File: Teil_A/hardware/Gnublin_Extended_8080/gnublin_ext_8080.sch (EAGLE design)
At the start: 7 parts

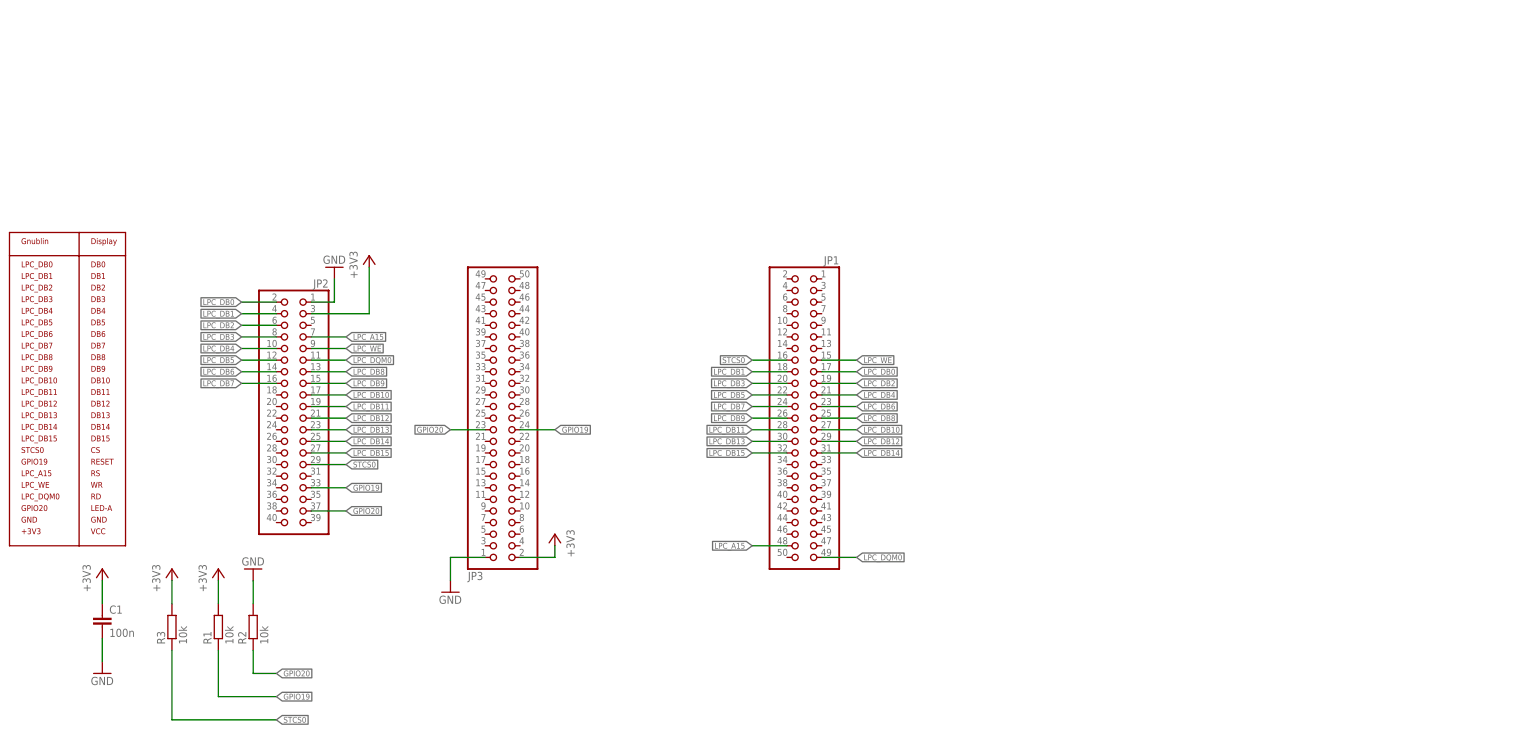
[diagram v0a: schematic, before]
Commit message: end of workday 29.07.2014
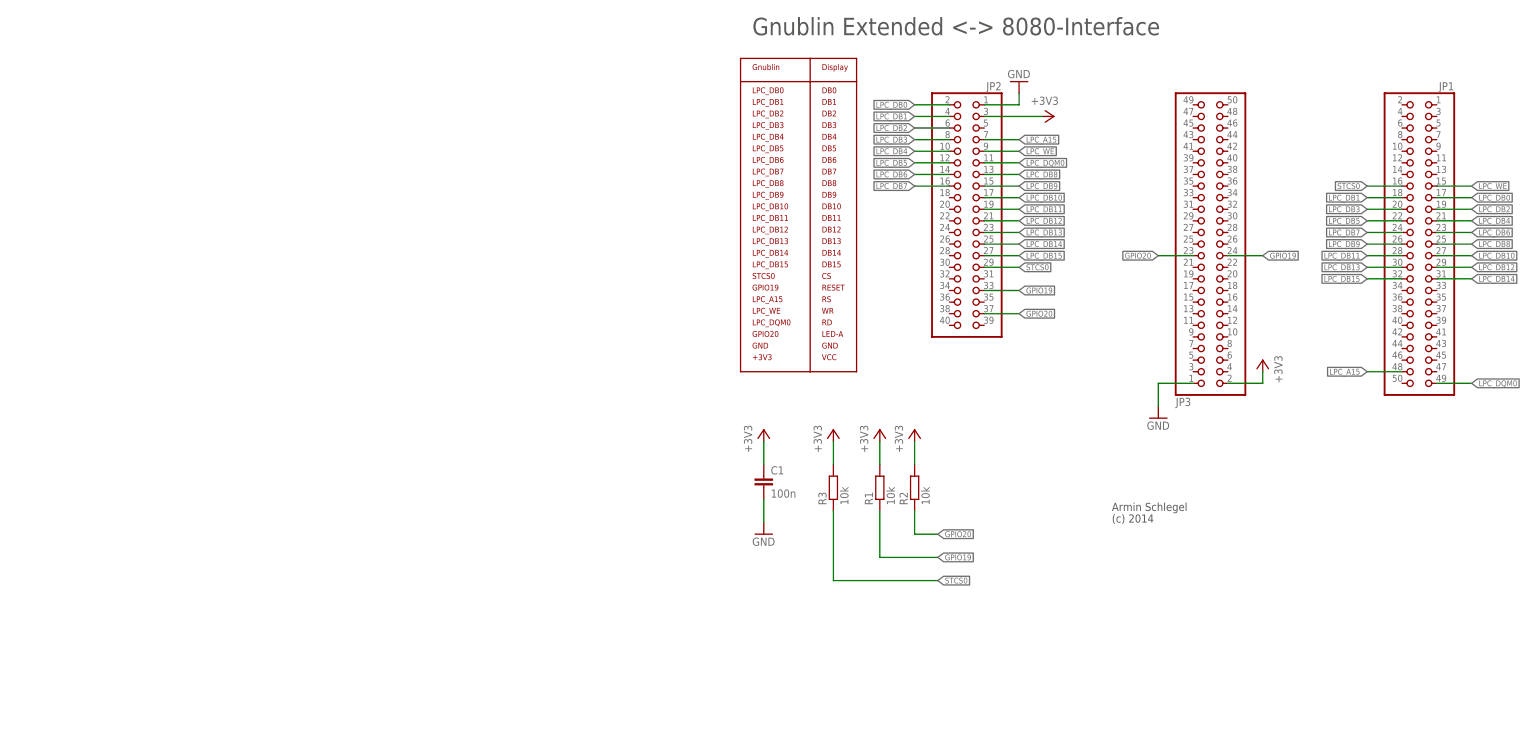
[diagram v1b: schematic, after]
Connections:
- net +3V3: now also R2.2
- net GND: no longer R2.2
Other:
- note added: "(c) 2014"
- note added: "Armin Schlegel"
- note added: "Gnublin Extended <-> 8080-Interface"
- moved on the sheet: C1, JP1, JP2, JP3, R1, R2, R3
